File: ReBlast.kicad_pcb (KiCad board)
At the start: 2 copper layers, 50.7 x 64.9 mm, 23 parts, among them J1 MOS_8580_Socket, U1 74HC20, U2 74HC139, U3 ZN428E-8, U4 TLC272, U5 MOS_8580, U6 ADC0804

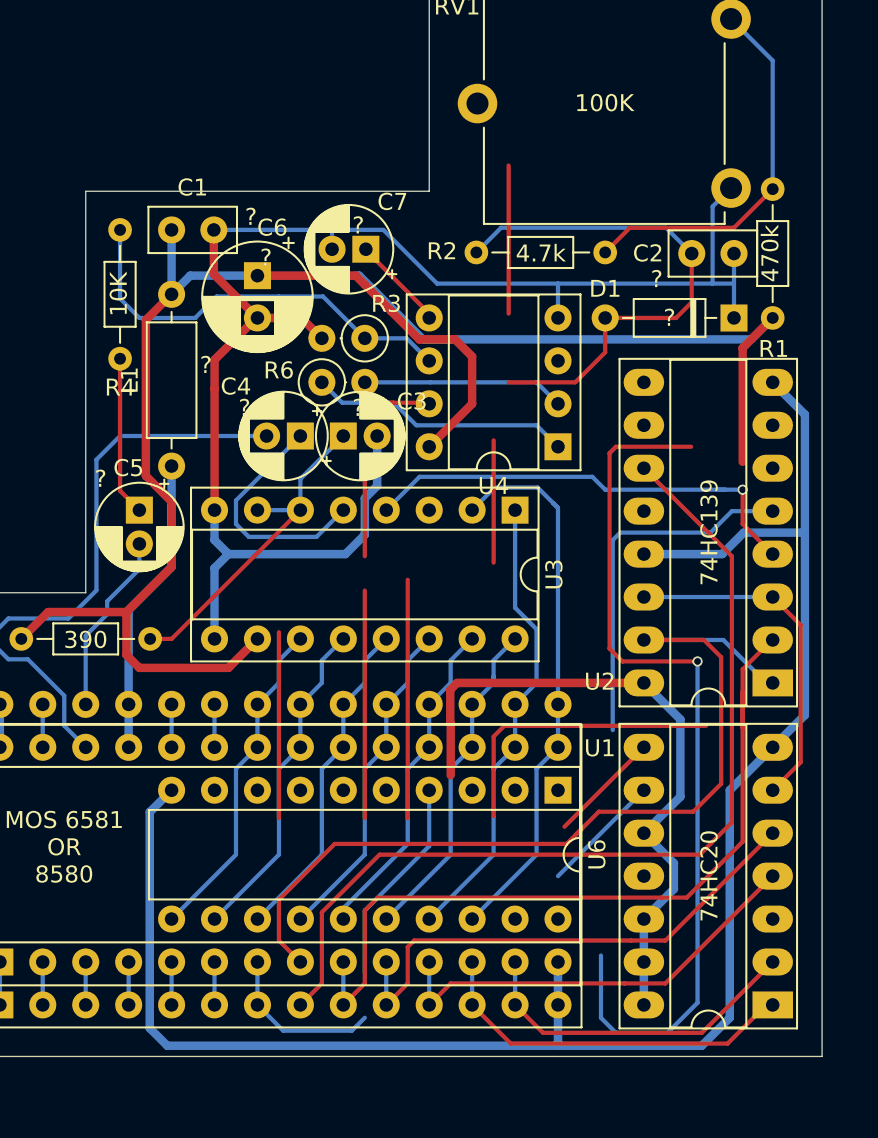
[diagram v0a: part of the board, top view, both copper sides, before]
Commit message: Done?
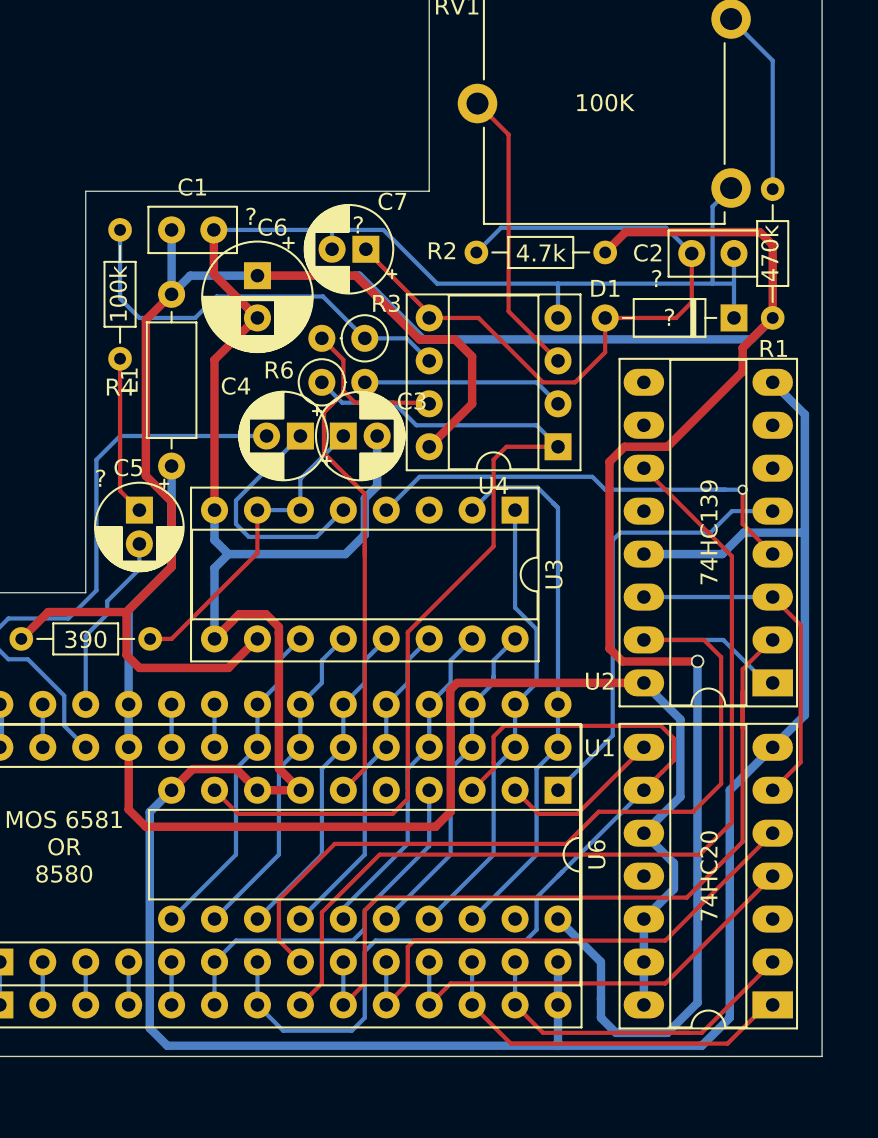
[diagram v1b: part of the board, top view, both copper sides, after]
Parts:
- C3: value 1u -> 4.7u
- C6: value 1u -> 47u
- R3, R6: value R -> 330k
- R4: value 10K -> 100k
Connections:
- C7 pad 1: Net-(C7-Pad1) -> Net-(C2-Pad1)
- R2 pad 1: Net-(R1-Pad2) -> +5V
- R3 pad 2: GNDA -> /adc_in
- R6 pad 1: Net-(R6-Pad1) -> /adc_vref_half
- U1 pad 10: +5V -> VCC
- U1 pad 12: +5V -> VCC
- U1 pad 13: +5V -> VCC
- U1 pad 14: +5V -> VCC
- U1 pad 8: Net-(U1-Pad8) -> /~read
- U1 pad 9: Net-(U1-Pad9) -> /r_~w
- U2 pad 16: +5V -> VCC
- U4 pad 1: Net-(R6-Pad1) -> /adc_vref_half
- U4 pad 3: Net-(U4-Pad3) -> Net-(RV1-Pad2)
- U4 pad 5: Net-(C7-Pad1) -> Net-(C2-Pad1)
- U4 pad 7: Net-(U4-Pad7) -> /adc_in
- U6 pad 2: Net-(U6-Pad2) -> /~read
- U6 pad 4: Net-(U6-Pad4) -> /phi2
- U6 pad 6: Net-(U6-Pad6) -> /adc_in
- U6 pad 7: Net-(U6-Pad7) -> GNDA
- U6 pad 8: Net-(U6-Pad8) -> GNDA
- U6 pad 9: Net-(U6-Pad9) -> /adc_vref_half
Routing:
- net (no net): track 130.1 -> 0.00 mm, vias 1 -> 0
- net VCC: track 17.7 -> 82.4 mm
- net /adc_vref_half: track 0.00 -> 54.2 mm
- net /r_~w: track 9.84 -> 54.4 mm
- net /adc_in: track 0.00 -> 35.5 mm
- net +5V: track 150.6 -> 181.9 mm, vias 0 -> 1
- net /phi2: track 2.54 -> 22.0 mm
- net GNDA: track 196.5 -> 215.8 mm
- net Net-(RV1-Pad2): track 0.00 -> 17.2 mm
- net Net-(R6-Pad1): track 15.5 -> 0.00 mm
- net Net-(U6-Pad4): track 12.4 -> 0.00 mm
- net Net-(C2-Pad1): track 30.9 -> 42.8 mm
- net Net-(R1-Pad2): track 22.5 -> 11.0 mm
- net /~read: track 0.00 -> 9.83 mm
- net Net-(U1-Pad9): track 7.18 -> 0.00 mm
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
